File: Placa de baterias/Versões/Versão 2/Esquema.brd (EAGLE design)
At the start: 41.9 x 28.6 mm, 7 parts

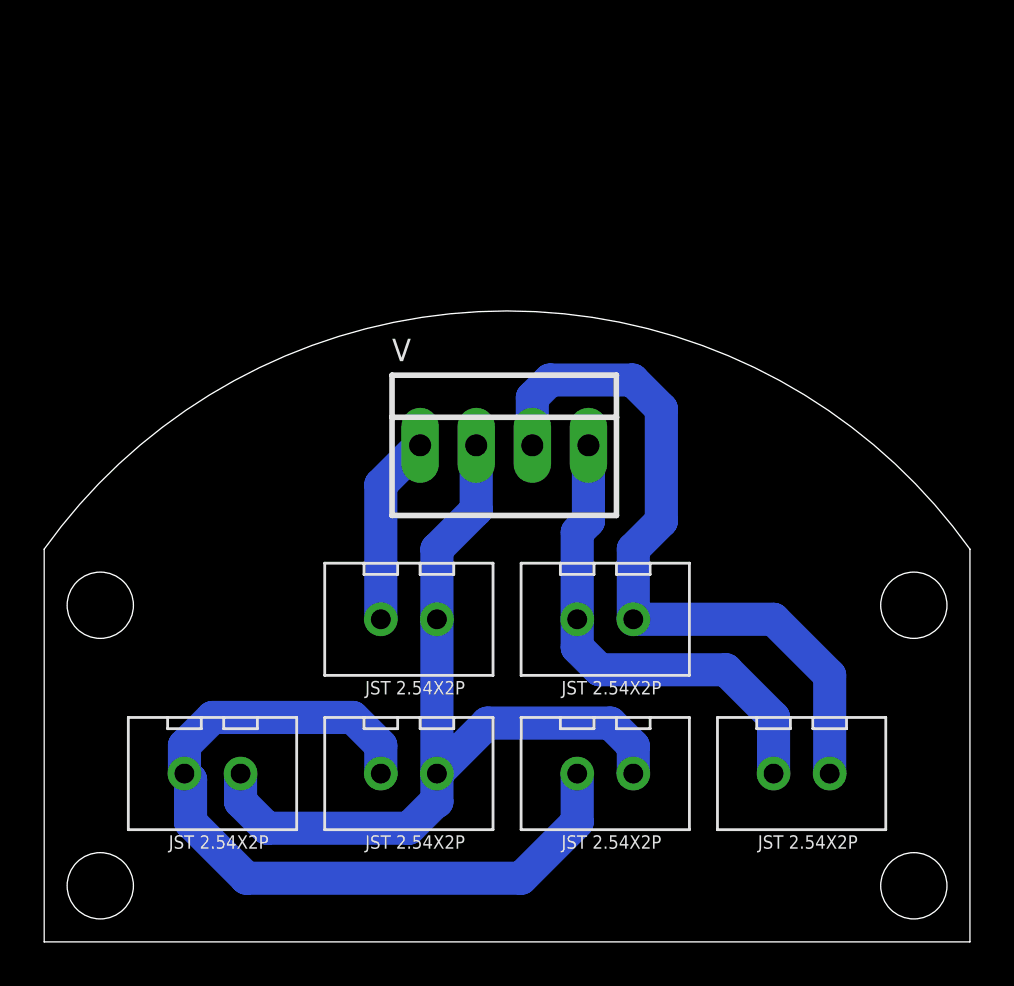
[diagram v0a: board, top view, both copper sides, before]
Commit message: placa de baterias
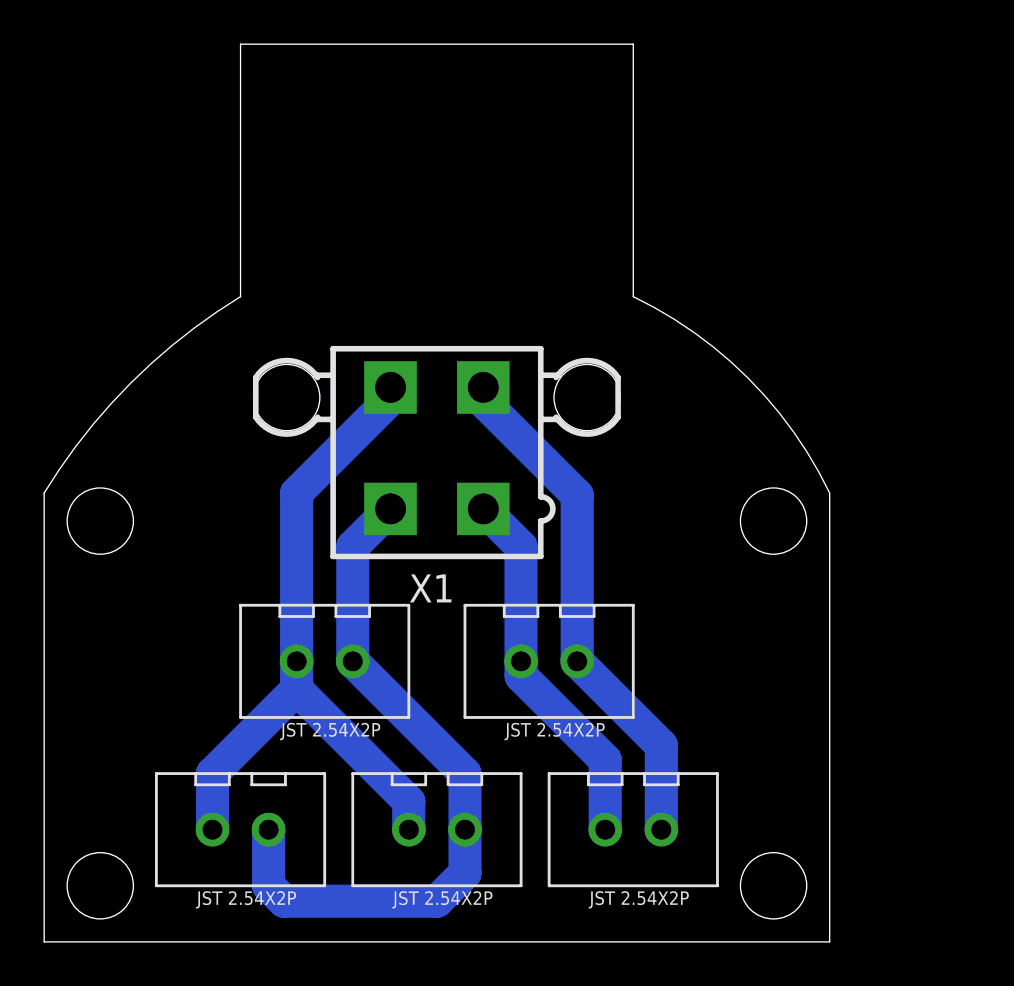
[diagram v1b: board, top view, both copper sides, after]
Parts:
- removed U$6: JST2.54X2P, CRD:JST2.54X2P_FOOTPRINT
- removed V: 22-23-2041, con-molex:22-23-2041
- added X1: 5566-4, con-molex:5566-4
- moved U$1 8.03 mm to (26.7, 5.08)
- moved U$5 4.26 mm to (12.7, 12.7)
- moved U$4 3.18 mm to (22.9, 12.7)
- moved U$3 2.84 mm to (8.89, 5.08)
- moved U$2 2.84 mm to (17.8, 5.08)
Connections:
- net V1+: now also X1.3; no longer V.3
- net V1-: now also X1.1; no longer V.4
- net V2+: now also X1.2; no longer U$6.1, V.2
- net V2-: now also X1.4; no longer U$6.2, V.1
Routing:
- net V2-: track 45.2 -> 31.8 mm
- net V1+: track 33.3 -> 23.4 mm
- net V2+: track 39.5 -> 31.5 mm
- net V1-: track 22.1 -> 16.8 mm
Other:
- board size 41.9 x 28.6 mm -> 35.6 x 40.6 mm
